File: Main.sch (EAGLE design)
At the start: 54 parts, among them IC1 LM75A, IC2 ADUM1400, IC3 74LS14N, Q1 IRF9530, U1 L298, U2 LM 1084 IT5,0, U3 LM 1084 IT3,3, U4 L298, X1 Motors, X3 Battery, X4 Ultra Sonics (5V), X5 ITG-3200, X6 PIRs

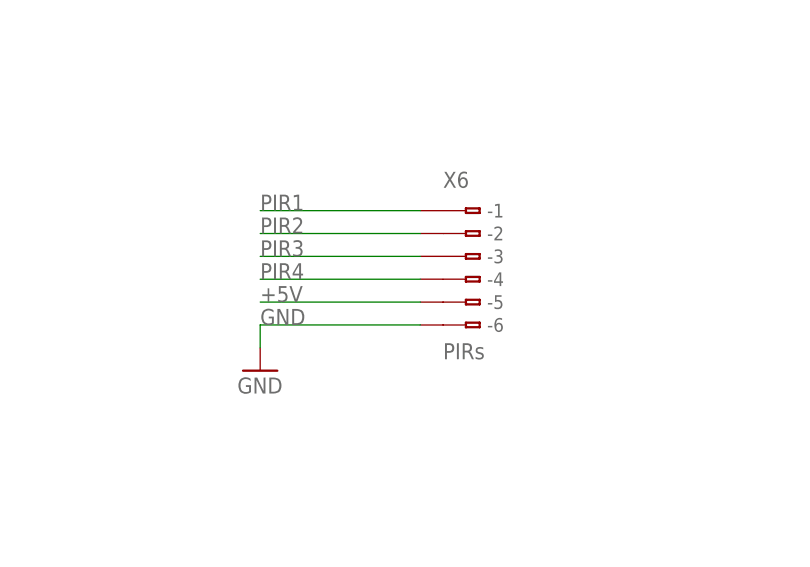
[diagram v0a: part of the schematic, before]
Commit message: optimizing board
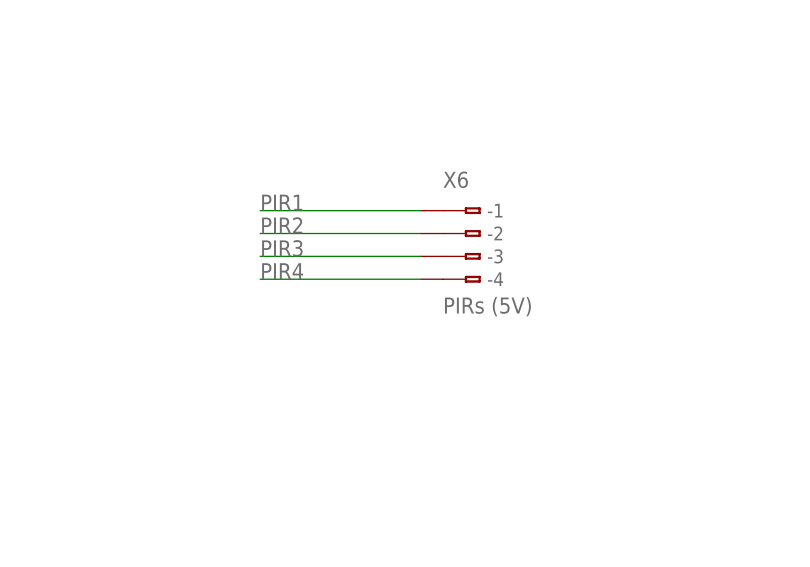
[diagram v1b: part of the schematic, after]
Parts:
- X6: value PIRs -> PIRs (5V); device con-wago:233-506 -> con-wago:233-504
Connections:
- net +5V: no longer X6.B-5
- net GND: no longer X6.B-6
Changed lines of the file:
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@@
 <part name="OK3" library="optocoupler" deviceset="PC847" device=""/>
 <part name="X5" library="con-wago" deviceset="233-504" device="" value="ITG-3200"/>
-<part name="X6" library="con-wago" deviceset="233-506" device="" value="PIRs"/>
-<part name="GND17" library="supply1" deviceset="GND" device=""/>
+<part name="X6" library="con-wago" deviceset="233-504" device="" value="PIRs (5V)"/>
 <part name="R10" library="resistor" deviceset="R-EU_" device="R0805" value="120"/>
 <part name="R11" library="resistor" deviceset="R-EU_" device="R0805" value="120"/>
@@
 <instance part="OK3" gate="D" x="-386.08" y="-302.26"/>
 <instance part="X5" gate="G$1" x="-441.96" y="-533.4"/>
-<instance part="X6" gate="G$1" x="-429.26" y="-15.24"/>
-<instance part="GND17" gate="1" x="-454.66" y="-27.94"/>
+<instance part="X6" gate="G$1" x="-429.26" y="-12.7"/>
 <instance part="R10" gate="G$1" x="-406.4" y="-246.38"/>
 <instance part="R11" gate="G$1" x="-406.4" y="-264.16"/>
@@
 <junction x="-457.2" y="513.08"/>
 <label x="-474.98" y="513.08" size="1.778" layer="95"/>
-</segment>
-<segment>
-<pinref part="X6" gate="G$1" pin="B-5"/>
-<wire x1="-436.88" y1="-20.32" x2="-454.66" y2="-20.32" width="0.1524" layer="91"/>
-<label x="-454.66" y="-20.32" size="1.778" layer="95"/>
 </segment>
 <segment>
@@
 </segment>
 <segment>
-<pinref part="X6" gate="G$1" pin="B-6"/>
-<wire x1="-436.88" y1="-22.86" x2="-454.66" y2="-22.86" width="0.1524" layer="91"/>
-<label x="-454.66" y="-22.86" size="1.778" layer="95"/>
-<pinref part="GND17" gate="1" pin="GND"/>
-<wire x1="-454.66" y1="-22.86" x2="-454.66" y2="-25.4" width="0.1524" layer="91"/>
-</segment>
-<segment>
